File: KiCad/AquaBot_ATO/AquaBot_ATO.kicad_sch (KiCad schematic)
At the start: 12 parts, among them M1 Motor_DC, Q1 IRLZ44N, Q2 IRLZ44N, U1 JTD2024S05

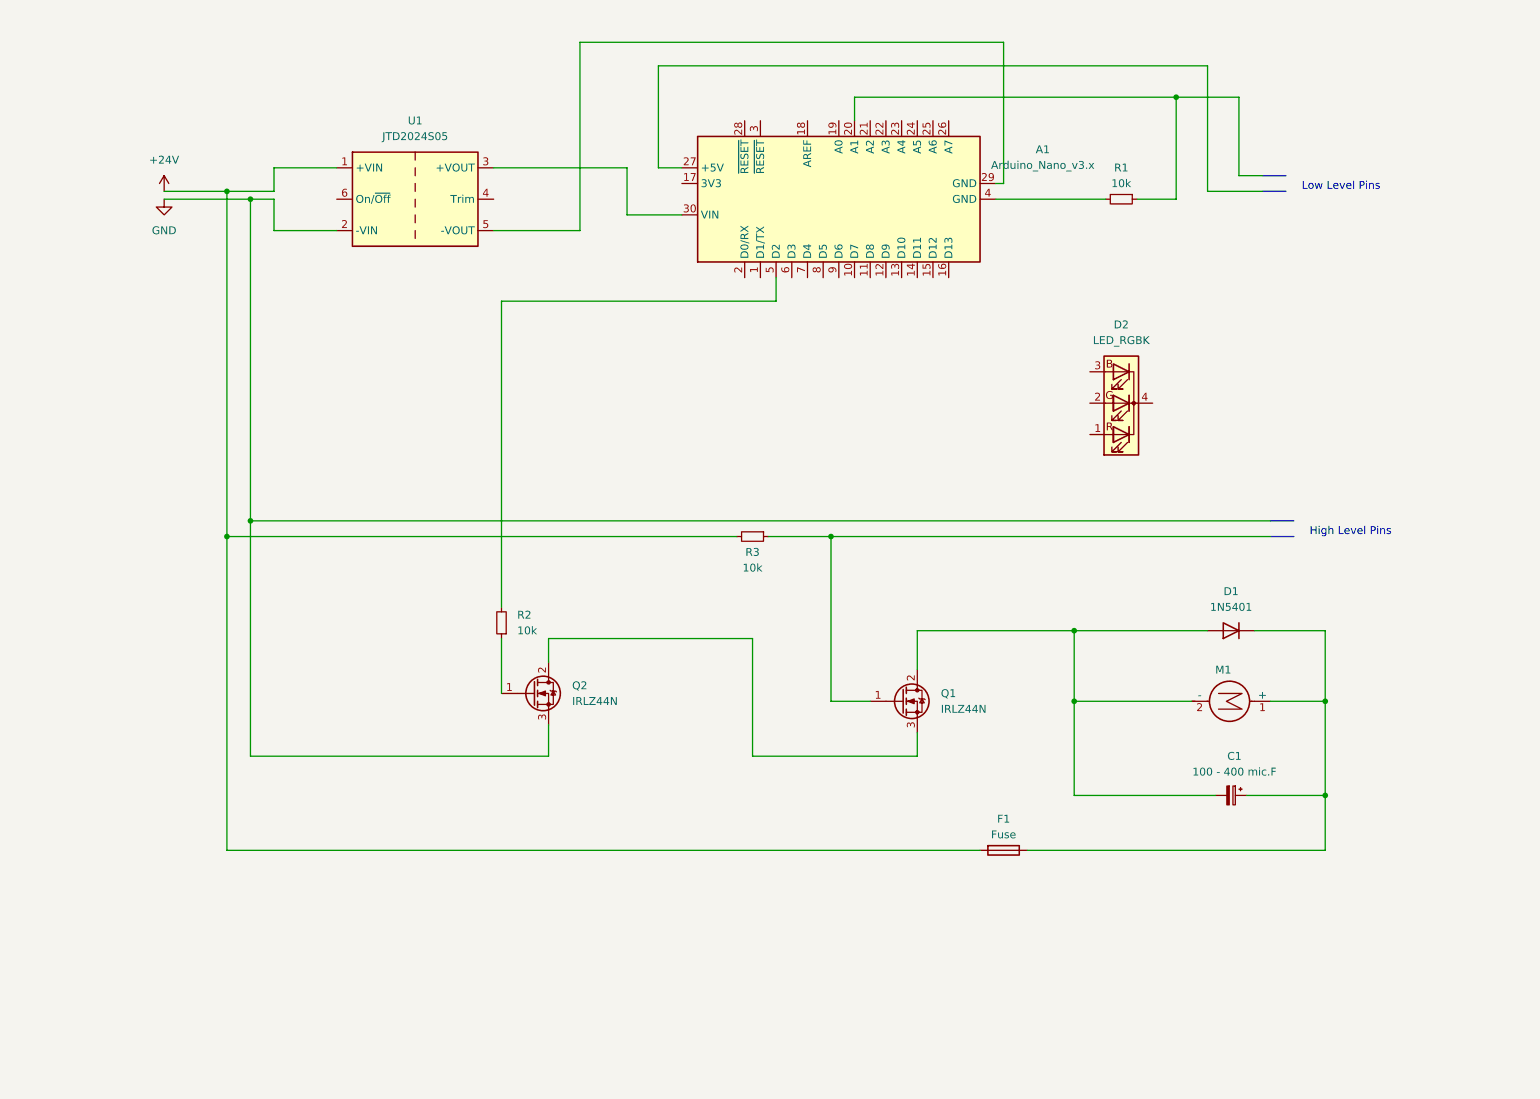
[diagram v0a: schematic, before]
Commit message: Improved the schematics and added a comment to the code
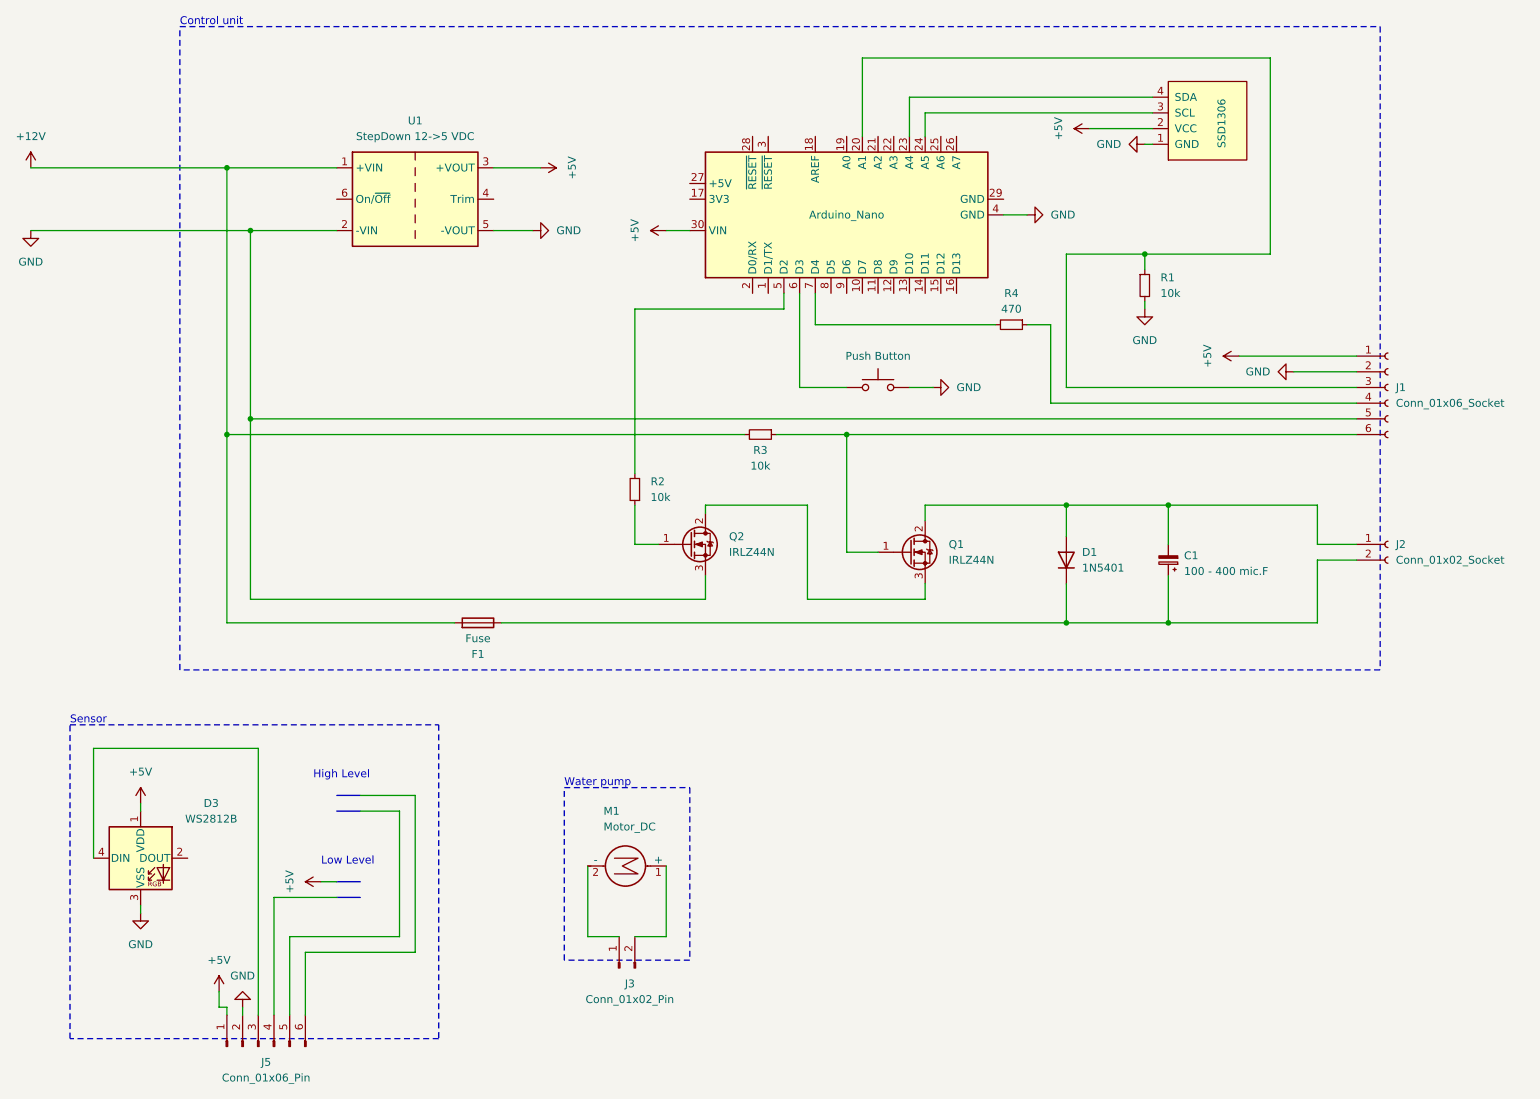
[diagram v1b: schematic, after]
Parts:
- removed D2: LED_RGBK, symbol Device:LED_RGBK
- added Brd1: SSD1306, symbol SSD1306-128x64_OLED:SSD1306
- added D3: WS2812B, LED_SMD:LED_WS2812B_PLCC4_5.0x5.0mm_P3.2mm, symbol LED:WS2812B
- added J1: Conn_01x06_Socket, symbol Connector:Conn_01x06_Socket
- added J2: Conn_01x02_Socket, symbol Connector:Conn_01x02_Socket
- added J3: Conn_01x02_Pin, symbol Connector:Conn_01x02_Pin
- added J5: Conn_01x06_Pin, symbol Connector:Conn_01x06_Pin
- added R4: 470, symbol Device:R_Small
- added SW1: Push Button, symbol Switch:SW_Push
- A1: value Arduino_Nano_v3.x -> Arduino_Nano
- U1: value JTD2024S05 -> StepDown 12->5 VDC
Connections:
- net GND: now also A1.4 (GND), R1.2, U1.5 (-VOUT), Brd1.1 (GND), D3.3 (VSS), J1.2 (Pin_2), J1.5 (Pin_5), J5.2 (Pin_2), SW1.2
- net at C1.1, D1.1 (K), F1.1: now also J2.2 (Pin_2); no longer M1.1 (+)
- net at C1.2, D1.2 (A), Q1.2 (D): now also J2.1 (Pin_1); no longer M1.2 (-)
- net +5V: now reaches A1.30 (VIN), U1.3 (+VOUT)
- net +5V: now also Brd1.2 (VCC), D3.1 (VDD), J1.1 (Pin_1), J5.1 (Pin_1)
- net at A1.29 (GND): no longer U1.5 (-VOUT)
- net at Q1.1 (G), R3.1: now also J1.6 (Pin_6)
- net at A1.20 (A1), R1.1: now also J1.3 (Pin_3)
- net at A1.23 (A4): now also Brd1.4 (SDA)
- net at A1.24 (A5): now also Brd1.3 (SCL)
- net at A1.6 (D3): now also SW1.1
- net at A1.7 (D4): now also R4.2
- net +24V renamed +12V
- new net: D3.4 (DIN), J5.3 (Pin_3)
- new net: J3.2 (Pin_2), M1.1 (+)
- new net: J3.1 (Pin_1), M1.2 (-)
- new net: J1.4 (Pin_4), R4.1
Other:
- note added: "Control unit"
- note added: "High Level"
- note added: "Low Level"
- note added: "Sensor"
- note added: "Water pump"
- note removed: "High Level Pins"
- note removed: "Low Level Pins"
- moved on the sheet: C1, D1, F1, Q1, Q2, R1, R2, R3
